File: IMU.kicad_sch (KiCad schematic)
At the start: 5 parts, among them U1 LSM6DS3TR-C

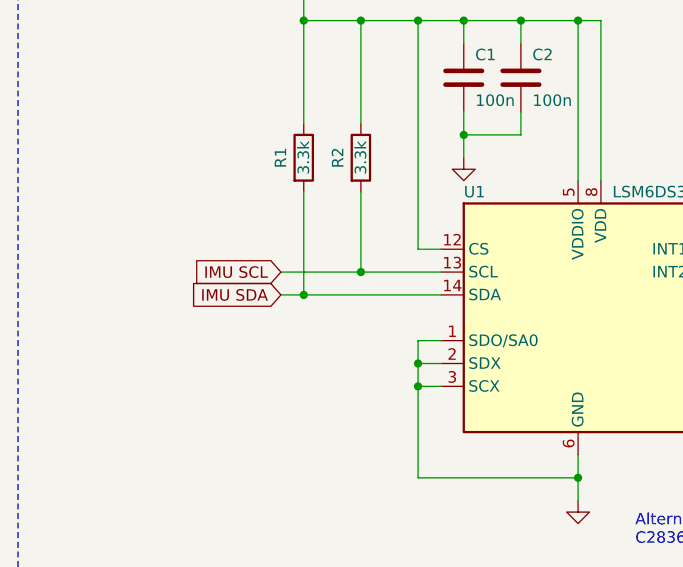
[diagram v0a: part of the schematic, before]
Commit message: initial
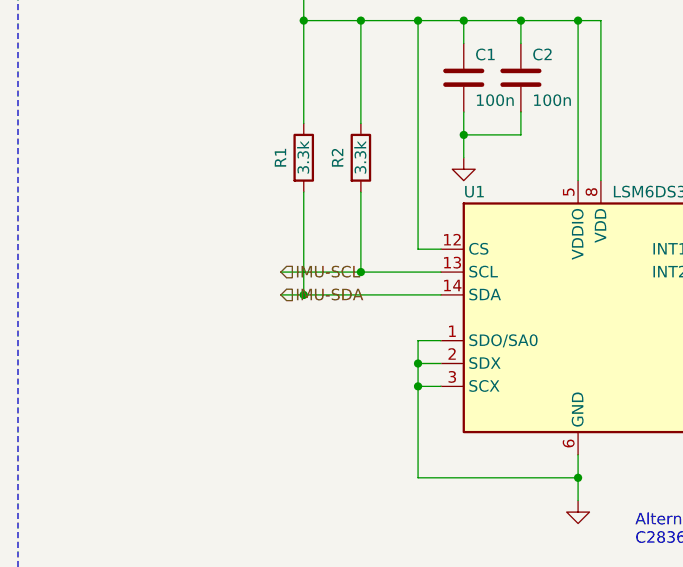
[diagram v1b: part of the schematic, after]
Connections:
- net IMU SCL renamed IMU-SCL
- net IMU SDA renamed IMU-SDA
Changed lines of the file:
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@@
 		)
 	)
-	(global_label "IMU SDA"
+	(hierarchical_label "IMU-SDA"
 		(shape input)
-		(at 106.68 105.41 180)
-		(fields_autoplaced yes)
+		(at 106.68 105.41 0)
 		(effects
 			(font
 				(size 1.27 1.27)
 			)
-			(justify right)
-		)
-		(property "Intersheetrefs" "${INTERSHEET_REFS}"
-			(at 96.506 105.41 0)
-			(hide yes)
-			(show_name no)
-			(do_not_autoplace no)
-			(effects
-				(font
-					(size 1.27 1.27)
-				)
-				(justify right)
-			)
+			(justify left bottom)
 		)
 	)
-	(global_label "IMU SCL"
+	(hierarchical_label "IMU-SCL"
 		(shape input)
-		(at 106.68 102.87 180)
-		(fields_autoplaced yes)
+		(at 106.68 102.87 0)
 		(effects
 			(font
 				(size 1.27 1.27)
 			)
-			(justify right)
-		)
-		(property "Intersheetrefs" "${INTERSHEET_REFS}"
-			(at 96.5665 102.87 0)
-			(hide yes)
-			(show_name no)
-			(do_not_autoplace no)
-			(effects
-				(font
-					(size 1.27 1.27)
-				)
-				(justify right)
-			)
+			(justify left bottom)
 		)
 	)
